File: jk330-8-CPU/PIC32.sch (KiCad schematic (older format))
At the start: 4 parts, among them U3001 PIC32MX795F512H, X3001 32.768khz

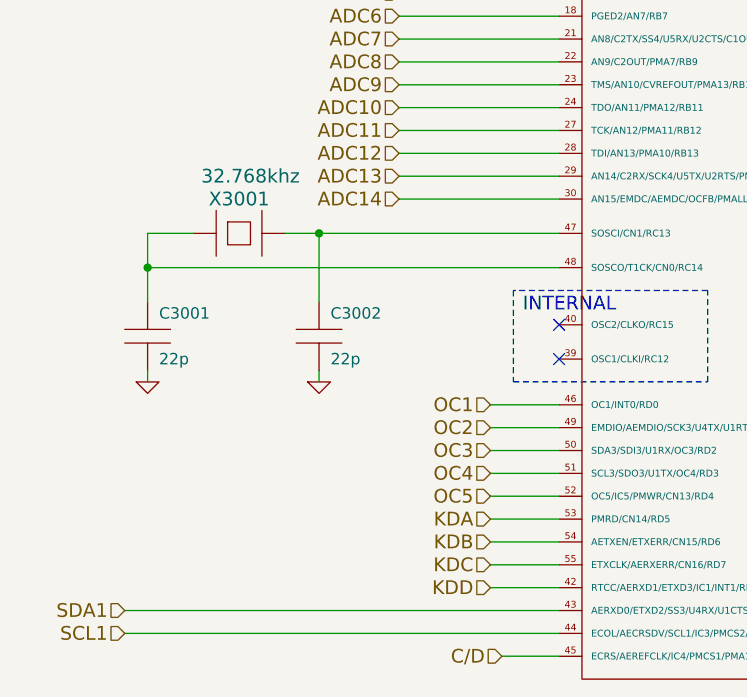
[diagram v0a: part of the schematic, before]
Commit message: CPU EN TEST
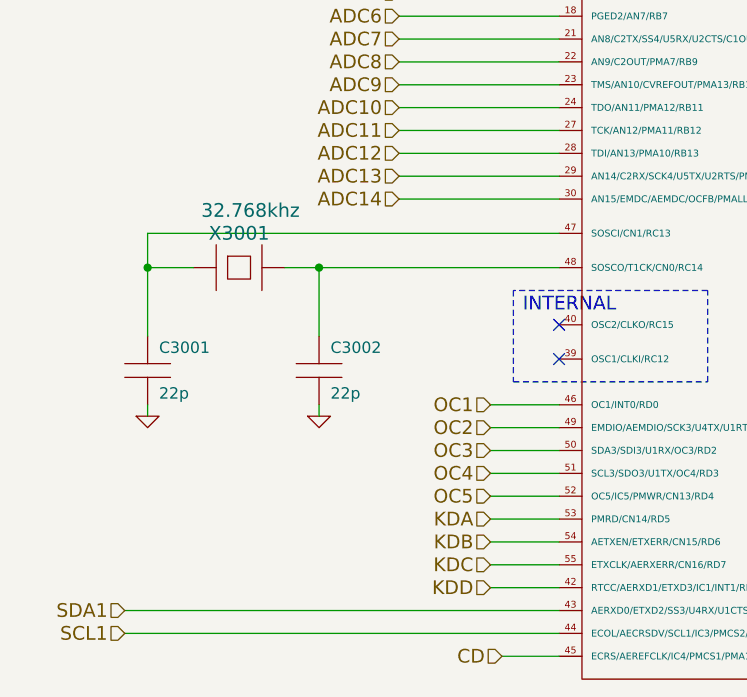
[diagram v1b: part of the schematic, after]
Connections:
- net at C3002.1, X3001.2: now also U3001.48 (SOSCO/T1CK/CN0/RC14); no longer U3001.47 (SOSCI/CN1/RC13)
- net at C3001.1, X3001.1: now also U3001.47 (SOSCI/CN1/RC13); no longer U3001.48 (SOSCO/T1CK/CN0/RC14)
- net C/D renamed CD
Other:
- moved on the sheet: C3001, C3002, X3001
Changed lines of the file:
@@
 Sheet 3 4
 Title "JK330-CPU"
-Date "24 sep 2013"
+Date "19 oct 2013"
 Rev "V1-00"
 Comp "F4DEB"
@@
 	7100 2400 7300 2400
 $Comp
-L GND #PWR093
+L GND #PWR094
 U 1 1 4FD220E7
 P 7300 2500
-F 0 "#PWR093" H 7300 2500 30  0001 C CNN
+F 0 "#PWR094" H 7300 2500 30  0001 C CNN
 F 1 "GND" H 7300 2430 30  0001 C CNN
 F 2 "" H 7300 2500 60  0001 C CNN
@@
 $EndComp
 $Comp
-L +3.3V #PWR094
+L +3.3V #PWR095
 U 1 1 4FD220DF
 P 7300 2400
-F 0 "#PWR094" H 7300 2360 30  0001 C CNN
+F 0 "#PWR095" H 7300 2360 30  0001 C CNN
 F 1 "+3.3V" H 7300 2510 30  0000 C CNN
 F 2 "" H 7300 2400 60  0001 C CNN
@@
 	4550 5750 4300 5750
 Text HLabel 4300 5750 0    60   Input ~ 0
-C/D
+CD
 Wire Wire Line
 	4550 2450 3850 2450
@@
 Wire Wire Line
 	3850 3750 4550 3750
-Wire Wire Line
-	3350 3900 4550 3900
 Wire Notes Line
 	4350 4150 4350 4550
@@
 Text HLabel 3850 3750 0    60   Input ~ 0
 ADC14
-Wire Wire Line
-	2750 4050 4550 4050
 $Comp
 L CRYSTAL1 X3001
 U 1 1 523F4EF1
-P 3150 3900
-F 0 "X3001" H 3150 4050 60  0000 C CNN
-F 1 "32.768khz" H 3200 4150 60  0000 C CNN
-F 2 "~" H 3150 3900 60  0000 C CNN
-F 3 "~" H 3150 3900 60  0000 C CNN
-	1    3150 3900
+P 3150 4050
+F 0 "X3001" H 3150 4200 60  0000 C CNN
+F 1 "32.768khz" H 3200 4300 60  0000 C CNN
+F 2 "~" H 3150 4050 60  0000 C CNN
+F 3 "~" H 3150 4050 60  0000 C CNN
+	1    3150 4050
 	1    0    0    -1
 $EndComp
@@
 L C C3001
 U 1 1 523F4F0A
-P 2750 4350
-F 0 "C3001" H 2800 4450 50  0000 L CNN
-F 1 "22p" H 2800 4250 50  0000 L CNN
-F 2 "~" H 2750 4350 60  0000 C CNN
-F 3 "~" H 2750 4350 60  0000 C CNN
-	1    2750 4350
+P 2750 4500
+F 0 "C3001" H 2800 4600 50  0000 L CNN
+F 1 "22p" H 2800 4400 50  0000 L CNN
+F 2 "~" H 2750 4500 60  0000 C CNN
+F 3 "~" H 2750 4500 60  0000 C CNN
+	1    2750 4500
 	1    0    0    -1
 $EndComp
@@
 L C C3002
 U 1 1 523F4F19
-P 3500 4350
-F 0 "C3002" H 3550 4450 50  0000 L CNN
-F 1 "22p" H 3550 4250 50  0000 L CNN
-F 2 "~" H 3500 4350 60  0000 C CNN
-F 3 "~" H 3500 4350 60  0000 C CNN
-	1    3500 4350
-	1    0    0    -1
-$EndComp
-Wire Wire Line
-	2750 3900 2750 4200
-Wire Wire Line
-	2750 3900 2950 3900
-Wire Wire Line
-	3500 4200 3500 3900
-Connection ~ 3500 3900
-Connection ~ 2750 4050
-Wire Wire Line
-	2750 4500 2750 4550
-Wire Wire Line
-	3500 4500 3500 4550
-$Comp
-L GND #PWR095
+P 3500 4500
+F 0 "C3002" H 3550 4600 50  0000 L CNN
+F 1 "22p" H 3550 4400 50  0000 L CNN
+F 2 "~" H 3500 4500 60  0000 C CNN
+F 3 "~" H 3500 4500 60  0000 C CNN
+	1    3500 4500
+	1    0    0    -1
+$EndComp
+Wire Wire Line
+	2750 3900 2750 4350
+Wire Wire Line
+	2750 4050 2950 4050
+Wire Wire Line
+	3500 4350 3500 4050
+Wire Wire Line
+	2750 4650 2750 4700
+Wire Wire Line
+	3500 4650 3500 4700
+$Comp
+L GND #PWR096
 U 1 1 523F514A
-P 2750 4550
-F 0 "#PWR095" H 2750 4550 30  0001 C CNN
-F 1 "GND" H 2750 4480 30  0001 C CNN
-F 2 "" H 2750 4550 60  0000 C CNN
-F 3 "" H 2750 4550 60  0000 C CNN
-	1    2750 4550
-	1    0    0    -1
-$EndComp
-$Comp
-L GND #PWR096
+P 2750 4700
+F 0 "#PWR096" H 2750 4700 30  0001 C CNN
+F 1 "GND" H 2750 4630 30  0001 C CNN
+F 2 "" H 2750 4700 60  0000 C CNN
+F 3 "" H 2750 4700 60  0000 C CNN
+	1    2750 4700
+	1    0    0    -1
+$EndComp
+$Comp
+L GND #PWR097
 U 1 1 523F5159
-P 3500 4550
-F 0 "#PWR096" H 3500 4550 30  0001 C CNN
-F 1 "GND" H 3500 4480 30  0001 C CNN
-F 2 "" H 3500 4550 60  0000 C CNN
-F 3 "" H 3500 4550 60  0000 C CNN
-	1    3500 4550
+P 3500 4700
+F 0 "#PWR097" H 3500 4700 30  0001 C CNN
+F 1 "GND" H 3500 4630 30  0001 C CNN
+F 2 "" H 3500 4700 60  0000 C CNN
+F 3 "" H 3500 4700 60  0000 C CNN
+	1    3500 4700
 	1    0    0    -1
 $EndComp
@@
 NoConn ~ 7100 4950
 NoConn ~ 7100 5050
+Wire Wire Line
+	3350 4050 4550 4050
+Connection ~ 3500 4050
+Wire Wire Line
+	4550 3900 2750 3900
+Connection ~ 2750 4050
 $EndSCHEMATC
